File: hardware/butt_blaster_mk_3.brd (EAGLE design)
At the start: 34 x 34 mm, 19 parts, among them Q1 2N3904, Q2 2N7000, Q3 2N3904, Q4 2N7000, Q5 2N7000

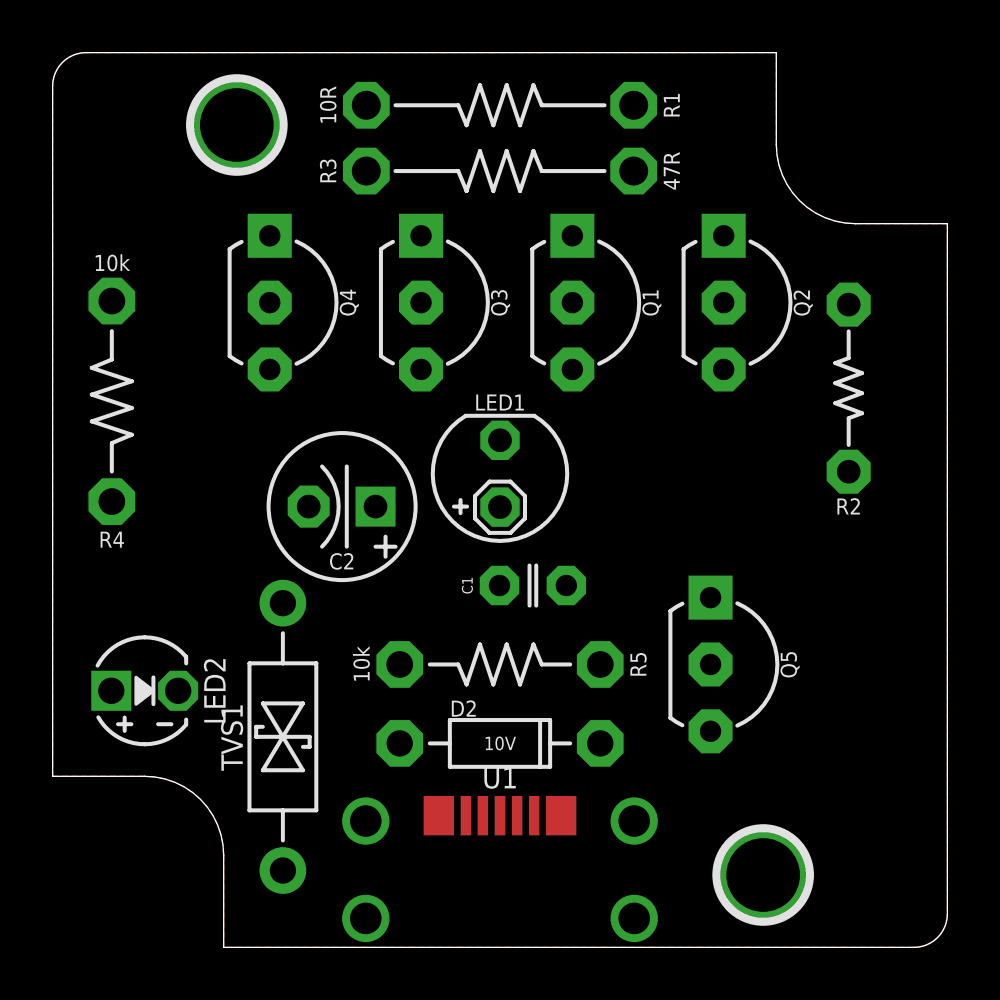
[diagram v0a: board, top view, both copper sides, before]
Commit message: huh
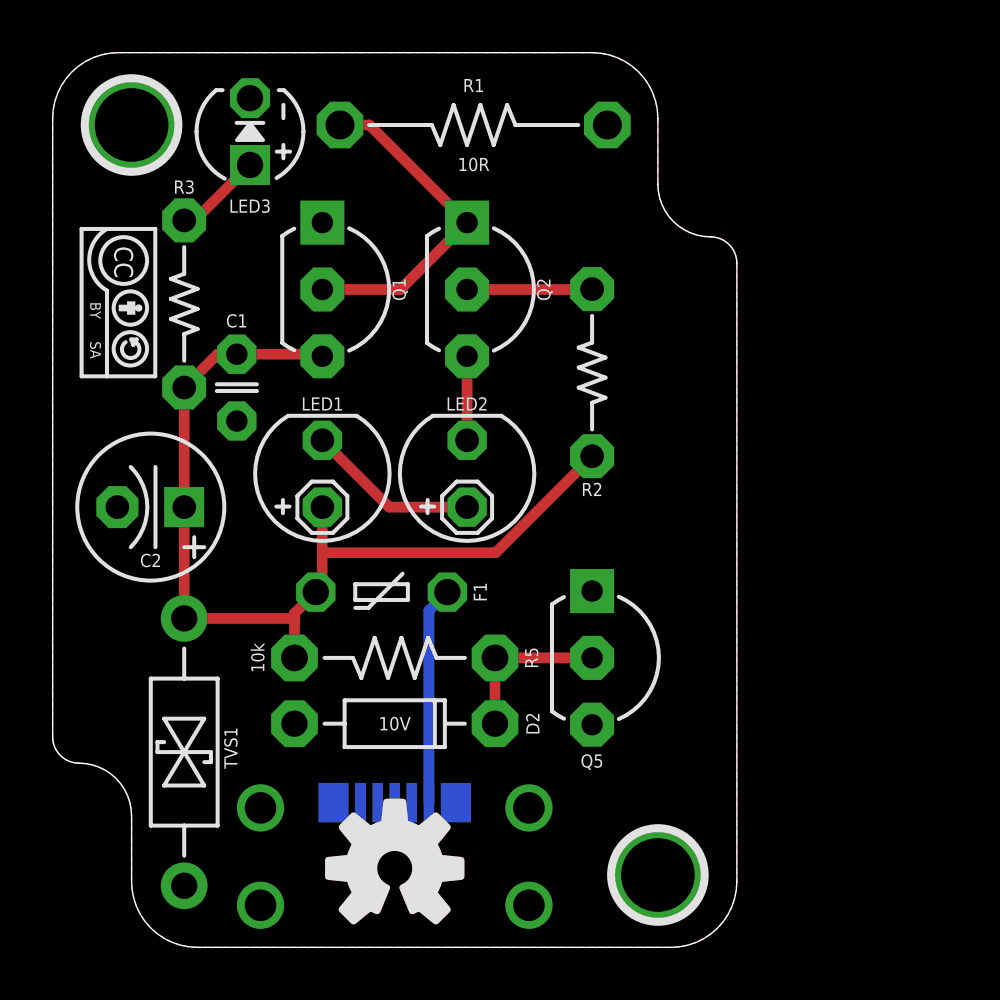
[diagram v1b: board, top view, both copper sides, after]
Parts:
- removed Q3: 2N3904, A_butts:TO-92-AMMO
- removed Q4: 2N7000, A_butts:TO-92-AMMO
- removed R4: 10k, A_butts:RESISTOR-AXIAL-PTH-7.68MM
- removed U1: (no value), A_butts:USB-MICRO-B-FCI-CUTOUT
- added F1: 250mA, A_butts:PTC
- added LED3: LED3MM, A_butts:LED3MM
- added PWR: (no value), A_butts:USB-MICRO-B-FCI-CUTOUT
- added U$2: (no value), A_butts:COW_SMALL
- added U$3, U$4: (no value), A_butts:CC-BY-SA-4.0-NO-URL
- added U$5: (no value), A_butts:OSHWLOGO_TOP_0.2_A
- LED2: value LED3MM -> LED5MM_SHORTPADS; device A_butts:LED3MM -> A_butts:LED5MM_SHORTPADS
- R3: value 47R -> 1k; device A_butts:RESISTOR-AXIAL-PTH-10.16MM -> A_butts:RESISTOR-AXIAL-PTH-6.35MM
- moved LED2 14.8 mm to (15.8, 18.0), turned to 90 degrees
- moved C1 13.5 mm to (7.00, 21.3), turned to 270 degrees
- moved R3 13.0 mm to (5.00, 24.4), turned to 270 degrees
- moved R2 9.77 mm to (20.5, 21.8)
- moved Q2 9.76 mm to (15.8, 25.0)
- moved Q1 9.51 mm to (10.2, 25.0)
- moved C2 7.27 mm to (3.73, 16.7)
- moved LED1 6.75 mm to (10.2, 18.0)
- moved Q5 4.51 mm to (20.5, 11.0)
- moved D2 4.07 mm to (13.0, 8.50)
- moved R5 4.01 mm to (13.0, 11.0)
- moved H1 4.00 mm to (3.00, 31.2)
- moved H2 4.00 mm to (23.0, 2.75)
- moved TVS1 3.79 mm to (5.00, 7.42)
- moved R1 1.25 mm to (16.0, 31.2), turned to 0 degrees
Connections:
- removed net N$9: D2.A, Q5.3, TVS1.P$1, U1.5, U1.P$1, U1.P$2
- new net REAL_GND: D2.A, PWR.5, PWR.P$1, PWR.P$2, Q5.3, TVS1.P$1
- net GND: now also LED3.K; no longer Q3.1, R3.P$2
- net N$1: now also LED2.A; no longer Q2.3
- net N$2: now also LED3.A; no longer Q3.2, Q4.1
- net N$3: now also LED2.K, Q2.3; no longer Q4.2, R4.P$2
- net N$4: now also F1.P$1, PWR.1; no longer LED2.K, Q4.3
- net VCC: now also F1.P$2, R3.P$2; no longer LED2.A, Q3.3, R4.P$1, U1.1
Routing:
- net VCC: track 0.00 -> 36.7 mm
- net N$6: track 0.00 -> 12.9 mm
- net N$4: track 0.00 -> 8.29 mm
- net N$1: track 0.00 -> 6.55 mm
- net N$5: track 0.00 -> 6.19 mm
- net N$8: track 0.00 -> 4.76 mm
- net N$2: track 0.00 -> 3.37 mm
- net N$3: track 0.00 -> 3.19 mm
- added copper zone on layer 16, net REAL_GND
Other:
- board size 34 x 34 mm -> 26 x 34 mm
